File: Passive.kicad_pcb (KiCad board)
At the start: 2 copper layers, 54.1 x 30.1 mm, 24 parts, among them J1 2.54 mm, J2 2.54 mm

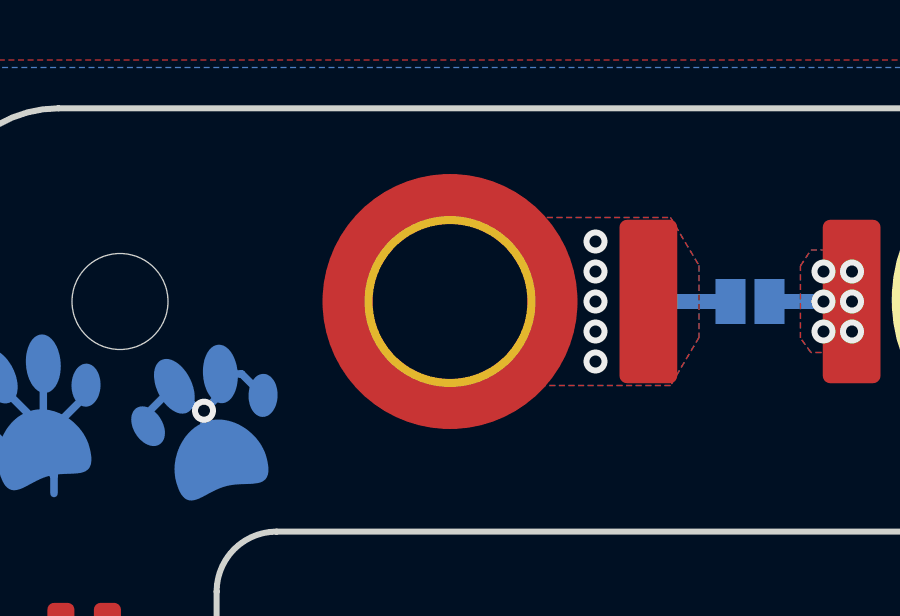
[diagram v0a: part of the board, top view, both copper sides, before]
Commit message: fixed a couple typos and improved readme
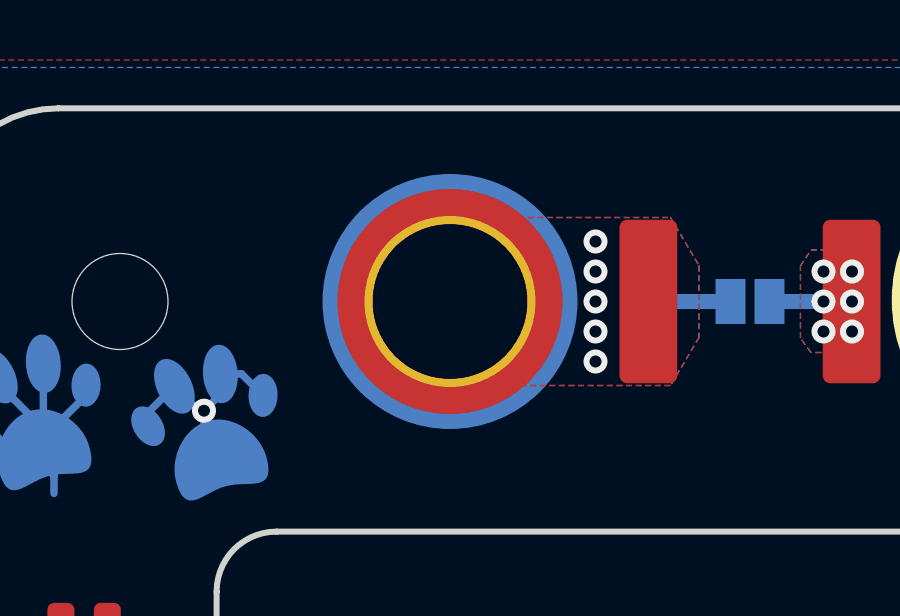
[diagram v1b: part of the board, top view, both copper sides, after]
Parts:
- H1: moved to B.Cu
- turned H1 to 180 degrees
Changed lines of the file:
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@@
     )
   )
-  (footprint "SamacSys_Parts:MountingHole_5.3mm_M5_DIN965_Pad_TopBottom" locked (layer "F.Cu")
-    (at 148.2 100.8)
-    (descr "Mounting Hole 5.3mm, M5, DIN965")
-    (tags "mounting hole 5.3mm m5 din965")
-    (property "Sheetfile" "Passive.kicad_sch")
-    (property "Sheetname" "")
-    (attr exclude_from_pos_files)
-    (fp_text reference "H1" (at 0 -5.6) (layer "F.SilkS") hide
-        (effects (font (size 1 1) (thickness 0.15)))
-    )
-    (fp_text value locked "575-4" (at 0 5.6) (layer "F.Fab")
-        (effects (font (size 1 1) (thickness 0.15)))
-    )
-    (fp_text user "${REFERENCE}" (at 0.3 0) (layer "F.Fab")
-        (effects (font (size 1 1) (thickness 0.15)))
-    )
-    (fp_circle (center 0 0) (end 4.1 0)
-      (stroke (width 0.15) (type solid)) (fill none) (layer "Cmts.User"))
-    (fp_circle (center 0 0) (end 4.85 0)
-      (stroke (width 0.05) (type solid)) (fill none) (layer "F.CrtYd"))
-    (pad "1" thru_hole circle locked (at 0 0) (size 5.7 5.7) (drill 5.16) (layers "*.Cu" "*.Mask")
-      (net 3 "Net-(F1-Pad2)") (pinfunction "1") (pintype "input"))
-    (pad "1" connect circle locked (at 0 0) (size 7.5 7.5) (layers "B.Cu" "B.Mask")
-      (net 3 "Net-(F1-Pad2)") (pinfunction "1") (pintype "input"))
-    (pad "1" connect circle locked (at 0 0) (size 8.5 8.5) (layers "F.Cu" "F.Mask")
-      (net 3 "Net-(F1-Pad2)") (pinfunction "1") (pintype "input"))
-    (model "P:/Electronic Projects/3D Models/575-4.step"
-      (offset (xyz 0 0 0))
-      (scale (xyz 1 1 1))
-      (rotate (xyz 0 0 0))
-    )
-  )
   (footprint "SamacSys_Parts:C_0603_1608Metric" (layer "F.Cu")
     (at 136.005 111.32)
@@
       (stroke (width 0) (type solid)) (fill solid) (layer "B.Mask"))
   )
+  (footprint "SamacSys_Parts:MountingHole_5.3mm_M5_DIN965_Pad_TopBottom" locked (layer "B.Cu")
+    (at 148.2 100.8 180)
+    (descr "Mounting Hole 5.3mm, M5, DIN965")
+    (tags "mounting hole 5.3mm m5 din965")
+    (property "Sheetfile" "Passive.kicad_sch")
+    (property "Sheetname" "")
+    (attr exclude_from_pos_files)
+    (fp_text reference "H1" (at 0 5.6) (layer "B.SilkS") hide
+        (effects (font (size 1 1) (thickness 0.15)) (justify mirror))
+    )
+    (fp_text value locked "575-4" (at 0 -5.6) (layer "B.Fab")
+        (effects (font (size 1 1) (thickness 0.15)) (justify mirror))
+    )
+    (fp_text user "${REFERENCE}" (at 0.3 0) (layer "B.Fab")
+        (effects (font (size 1 1) (thickness 0.15)) (justify mirror))
+    )
+    (fp_circle (center 0 0) (end 4.1 0)
+      (stroke (width 0.15) (type solid)) (fill none) (layer "Cmts.User"))
+    (fp_circle (center 0 0) (end 4.85 0)
+      (stroke (width 0.05) (type solid)) (fill none) (layer "B.CrtYd"))
+    (pad "1" thru_hole circle locked (at 0 0 180) (size 5.7 5.7) (drill 5.16) (layers "*.Cu" "*.Mask")
+      (net 3 "Net-(F1-Pad2)") (pinfunction "1") (pintype "input"))
+    (pad "1" connect circle locked (at 0 0 180) (size 7.5 7.5) (layers "F.Cu" "F.Mask")
+      (net 3 "Net-(F1-Pad2)") (pinfunction "1") (pintype "input"))
+    (pad "1" connect circle locked (at 0 0 180) (size 8.5 8.5) (layers "B.Cu" "B.Mask")
+      (net 3 "Net-(F1-Pad2)") (pinfunction "1") (pintype "input"))
+    (model "P:/Electronic Projects/3D Models/575-4.step"
+      (offset (xyz 0 0 0))
+      (scale (xyz 1 1 1))
+      (rotate (xyz 0 0 0))
+    )
+  )
   (footprint "KiCAD Library:pawpad_holeless" (layer "B.Cu")
